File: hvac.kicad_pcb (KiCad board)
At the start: 2 copper layers, 191.8 x 114.3 mm, 44 parts, among them IC1 ATMEGA328P-A, J1 PROGRAMMING HEADER, J2 SERIAL PORT, J3 POWER_INPUT, SW1 SPST, SW2 SPST, SW3 SPST, U1 MIC5225, U2 MOSFET_N, U3 MOSFET_N, U4 MOSFET_N

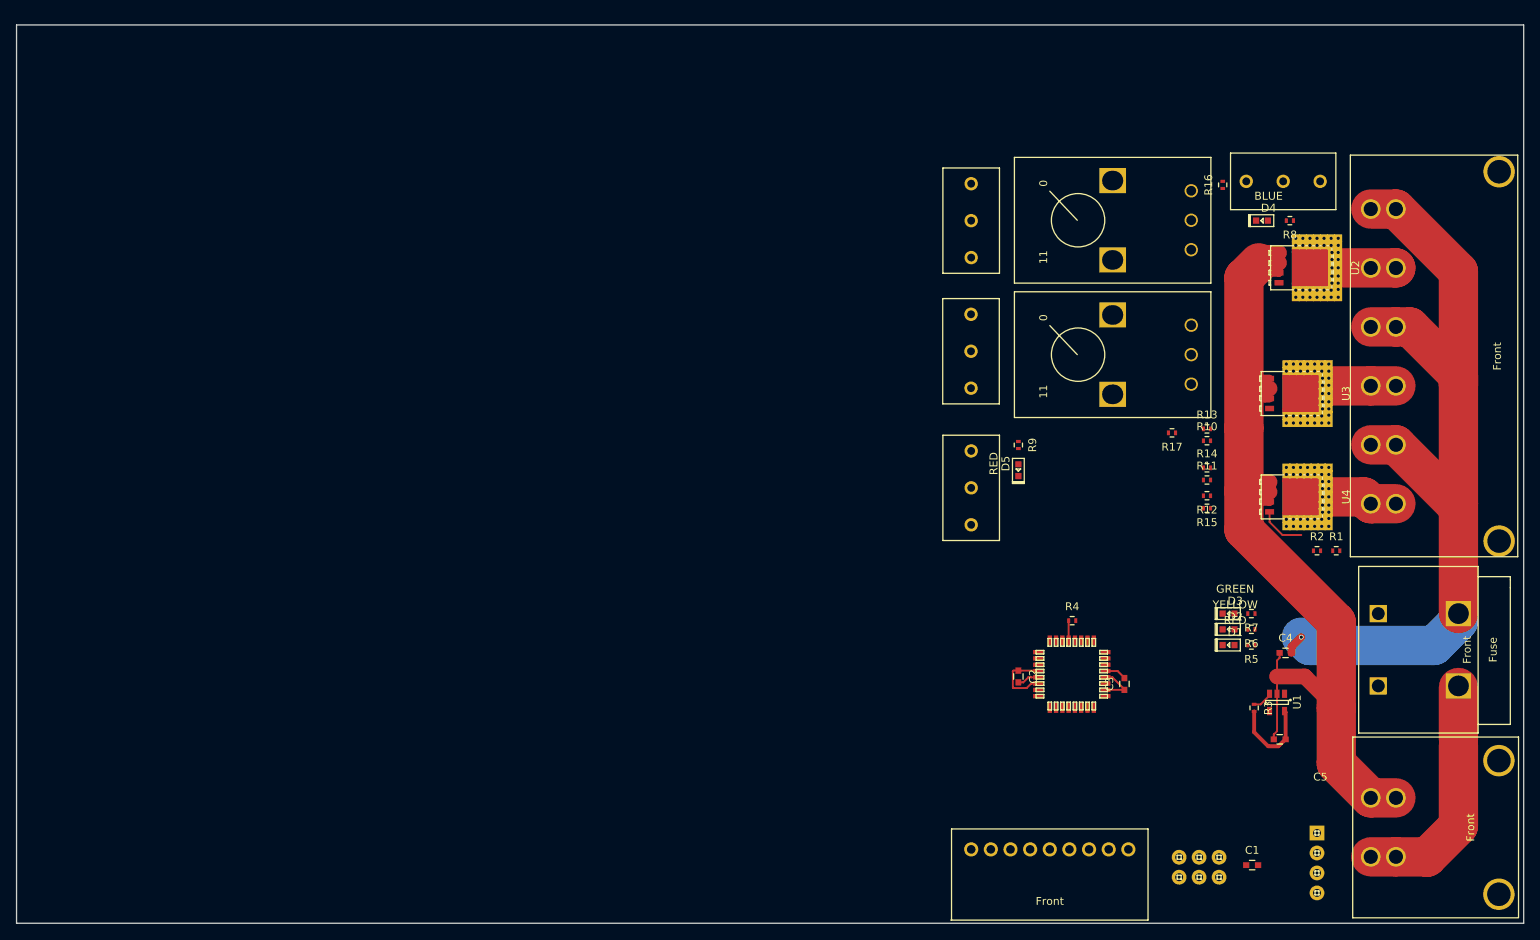
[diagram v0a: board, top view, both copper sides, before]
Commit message: Add holes to the pcb layout
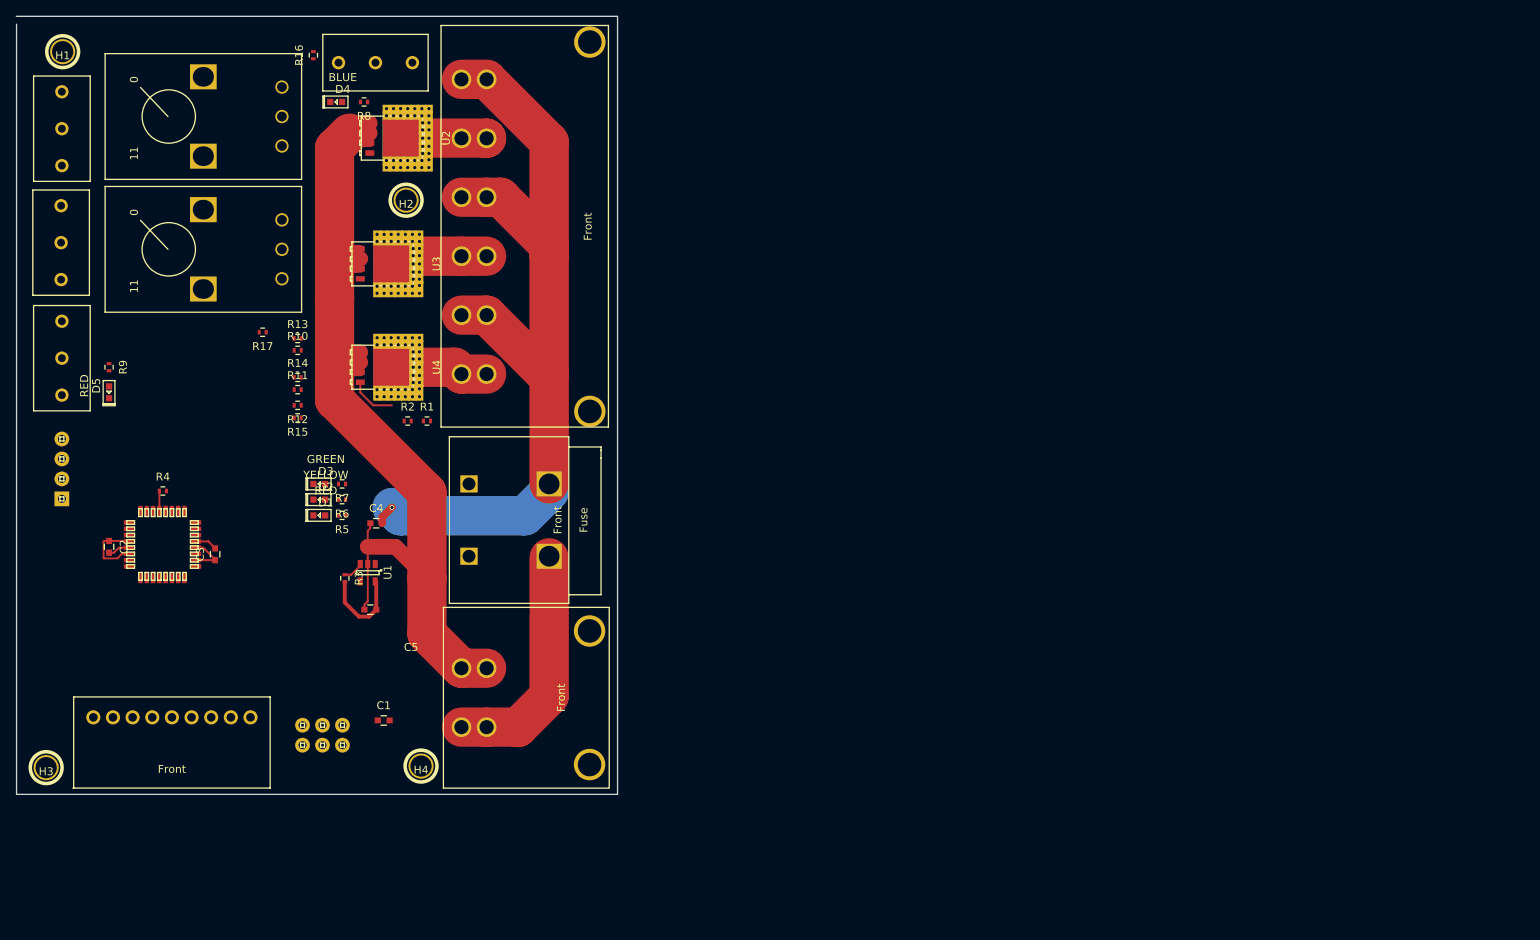
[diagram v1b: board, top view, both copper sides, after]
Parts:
- added H1: hole, homebrew:hole-m2.5, F.Cu at (55.4, 41.5)
- added H2: hole, homebrew:hole-m2.5, F.Cu at (99.1, 60.4)
- added H3: hole, homebrew:hole-m2.5, F.Cu at (53.3, 132.6)
- added H4: hole, homebrew:hole-m2.5, F.Cu at (101.0, 132.4)
- moved J2 165.3 mm to (55.3, 98.4), turned to 90 degrees
- moved R8 118.8 mm to (93.8, 47.9)
- moved D4 118.8 mm to (90.2, 47.9)
- moved J3 116.9 mm to (109.3, 123.7)
- moved JP1 116.9 mm to (109.3, 63.8)
- moved U3 116.9 mm to (96.1, 68.5)
- moved U4 116.9 mm to (96.1, 81.7)
- moved C2 116.9 mm to (61.3, 104.5)
- moved C3 116.9 mm to (74.8, 105.5)
- moved C4 116.9 mm to (95.3, 101.5)
- moved C5 116.9 mm to (94.5, 112.5)
- moved D1 116.9 mm to (88.0, 100.5)
- moved D2 116.9 mm to (88.0, 98.5)
- moved D3 116.9 mm to (88.0, 96.5)
- moved F1 116.9 mm to (112.2, 101.1)
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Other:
- board size 191.8 x 114.3 mm -> 76.5 x 99 mm
